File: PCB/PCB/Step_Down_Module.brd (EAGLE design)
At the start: 191.8 x 104.1 mm, 42 parts, among them Q1 TPH2900ENH

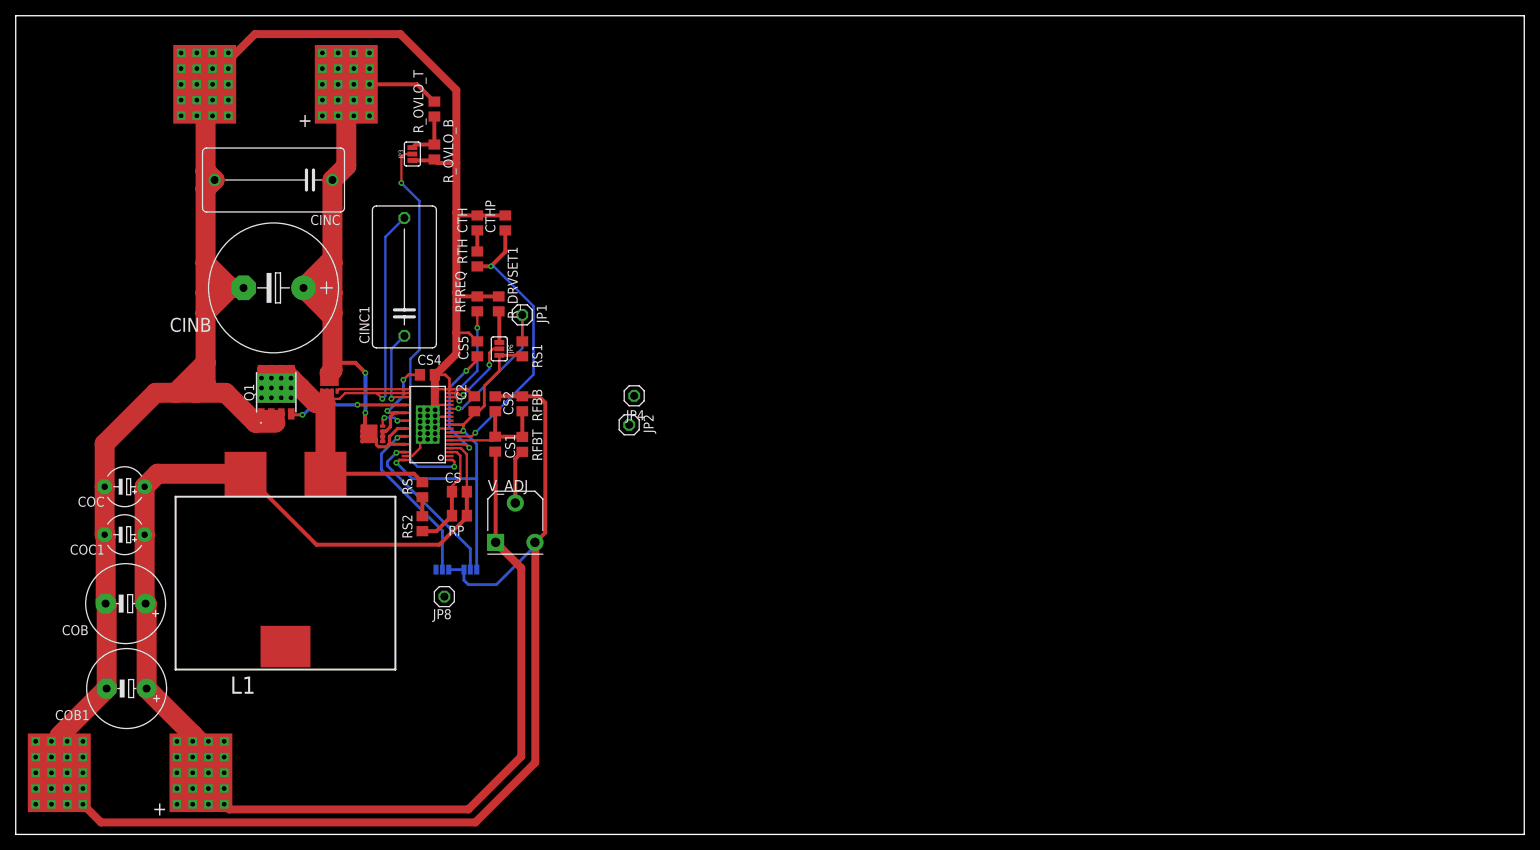
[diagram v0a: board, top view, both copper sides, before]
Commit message: Finalized PCB - first iteration
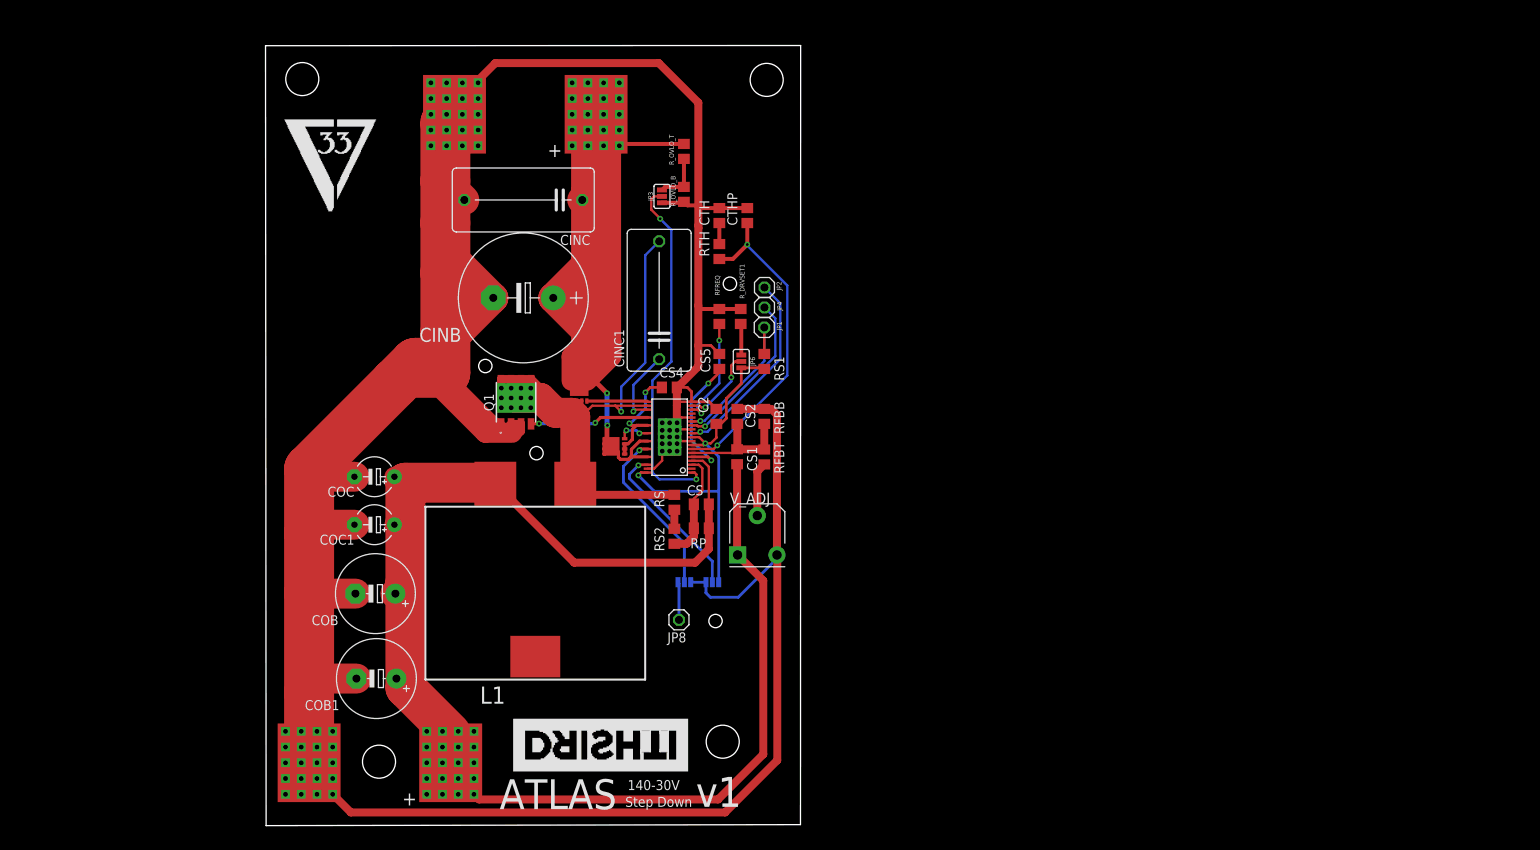
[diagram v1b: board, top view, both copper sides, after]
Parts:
- moved CINC1 32.5 mm to (50.0, 66.4)
- moved R_OVLO_B 32.2 mm to (53.2, 79.8)
- moved R_OVLO_T 32.2 mm to (53.2, 85.3)
- moved JP3 32.2 mm to (50.4, 79.6)
- moved RS2 32.1 mm to (52.0, 36.4)
- moved RS 32.1 mm to (52.0, 40.7)
- moved U$5 32.0 mm to (33.0, 87.6)
- moved CINC 31.9 mm to (32.8, 79.1)
- moved CINB 31.8 mm to (32.8, 66.7)
- moved COB 31.8 mm to (14.0, 29.1)
- moved COB1 31.8 mm to (14.1, 18.3)
- moved COC 31.8 mm to (13.8, 43.9)
- moved COC1 31.8 mm to (13.8, 37.8)
- moved L1 31.8 mm to (34.3, 28.7)
- moved U$3 31.8 mm to (39.9, 54.6)
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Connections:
- net GND: now also U$1.39_B; no longer U$1.PWR_PAD16, U$1.PWR_PAD17, U$1.PWR_PAD18
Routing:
- net GND: track 522.7 -> 603.6 mm
- net CLKOUT: track 0.00 -> 25.1 mm, vias 0 -> 1
- net PLLIN: track 0.00 -> 21.3 mm, vias 0 -> 1
- net N$3: track 99.7 -> 92.4 mm
- net N$13: track 0.00 -> 4.83 mm
- net ITH: track 37.2 -> 41.8 mm
- net OVLO: track 48.8 -> 45.6 mm
- net VOUT: track 181.0 -> 178.9 mm
- net VIN: track 98.8 -> 97.7 mm
- net INTVCC: track 49.2 -> 50.2 mm
- net N$8: track 16.4 -> 15.4 mm
- net N$1: track 8.83 -> 8.12 mm
- net N$4: track 10.6 -> 9.91 mm
- net N$6: track 14.2 -> 13.5 mm
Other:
- board size 191.8 x 104.1 mm -> 68 x 99.2 mm
- board text added: "140-30V"
- board text added: "ATLAS"
- board text added: "Step Down"
- board text added: "v1"
